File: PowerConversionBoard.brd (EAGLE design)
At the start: 152.4 x 76.2 mm, 48 parts, among them U1 LM2678, U2 LM2678

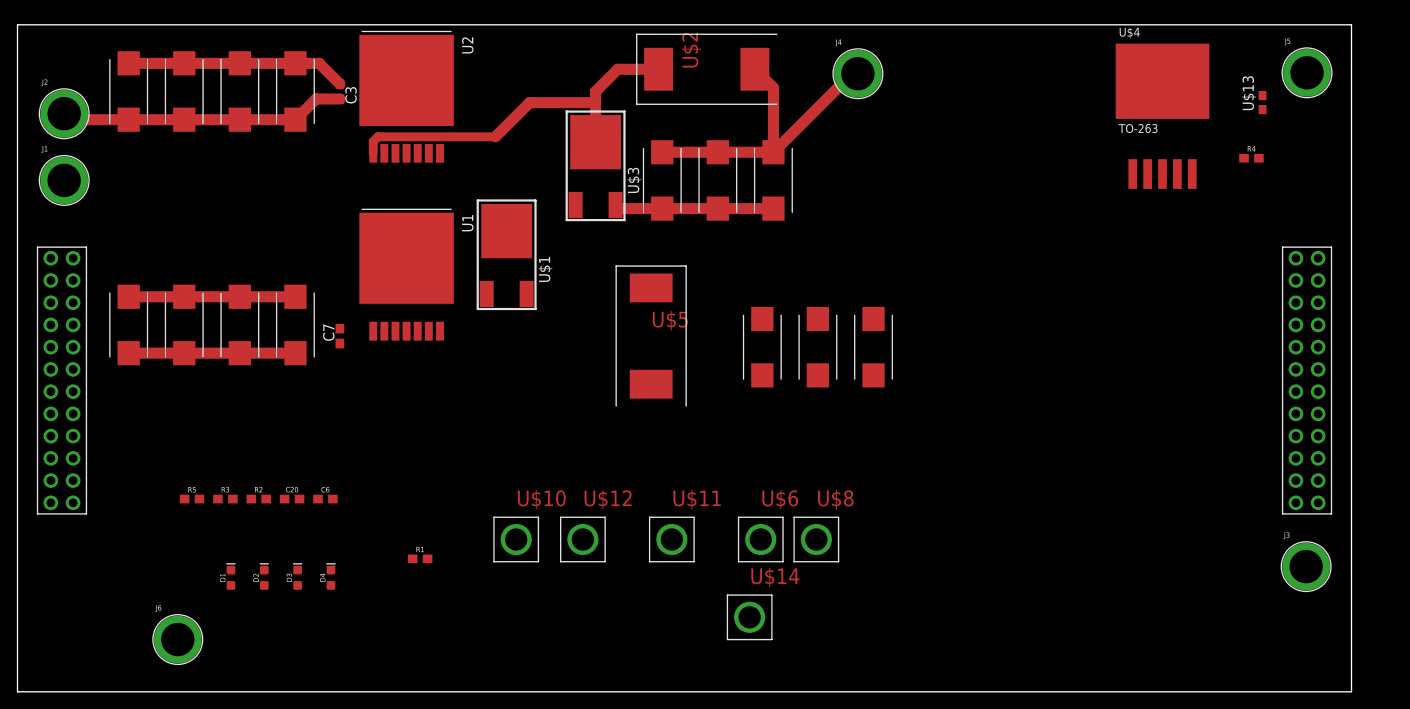
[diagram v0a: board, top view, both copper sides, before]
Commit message: Did some stuff
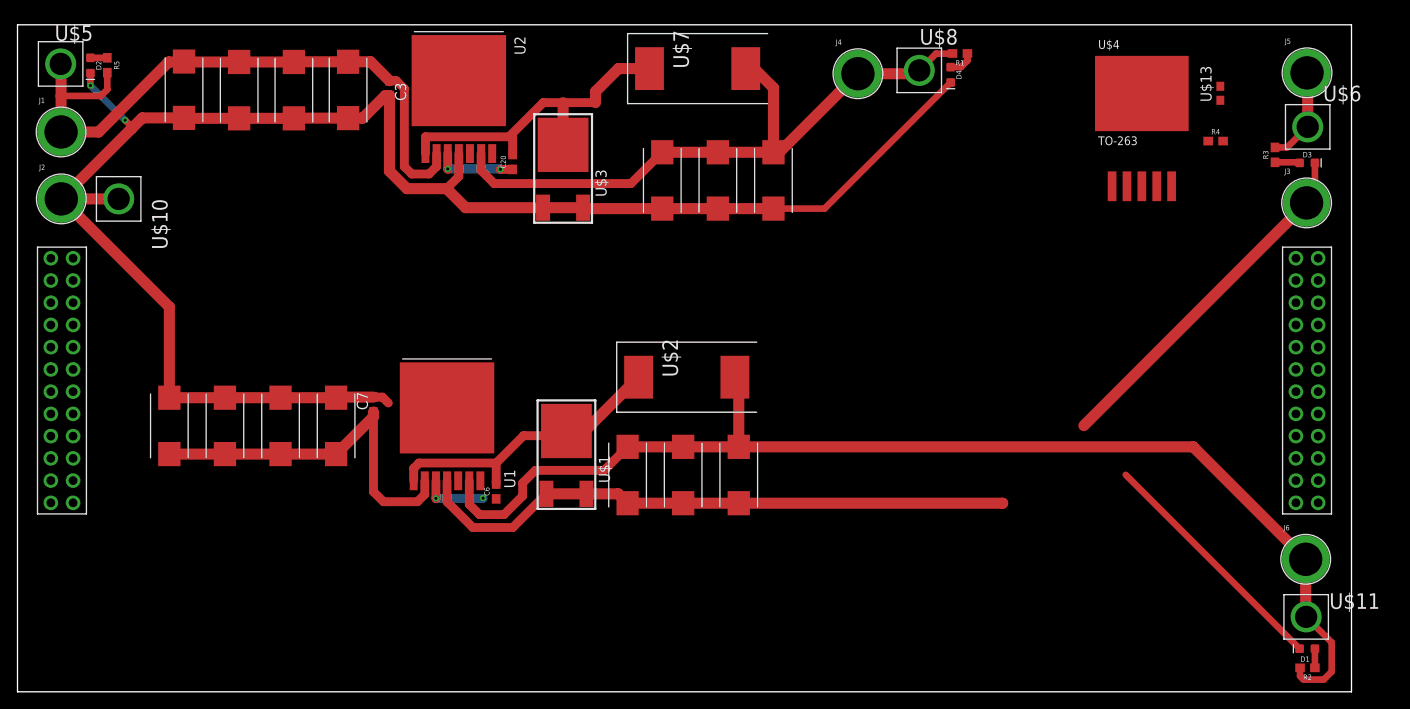
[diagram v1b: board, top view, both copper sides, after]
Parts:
- removed U$12, U$14: TP, TP:TP
- added U$7: HCM1305, HCM1305:HCM1305
- U$5: value HCM1305 -> TP; device HCM1305:HCM1305 -> TP:TP
- moved J6 129.2 mm to (147.2, 15.1)
- moved R3 126.2 mm to (143.7, 61.3), turned to 90 degrees
- moved D3 124.7 mm to (147.3, 60.4), turned to 0 degrees
- moved D1 123.2 mm to (147.3, 4.93), turned to 180 degrees
- moved R2 121.4 mm to (147.4, 2.74), turned to 180 degrees
- moved D4 91.2 mm to (106.6, 70.5), turned to 270 degrees
- moved R1 84.5 mm to (107.7, 72.9), turned to 180 degrees
- moved U$6 78.3 mm to (147.4, 64.5)
- moved U$5 74.3 mm to (4.93, 71.7)
- moved U$11 73.0 mm to (147.2, 8.56)
- moved D2 61.8 mm to (8.33, 71.6), turned to 270 degrees
- moved U$10 59.8 mm to (11.6, 56.3), turned to 270 degrees
- moved U$8 54.9 mm to (103.0, 71.0)
- moved R5 50.5 mm to (10.3, 71.6), turned to 270 degrees
- moved C20 46.0 mm to (56.6, 60.5), turned to 90 degrees
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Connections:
- net +12V: now also U$5.P$1; no longer U$12.P$1, U$14.P$1
- net +5V: now also U$11.P$1, U$2.2; no longer U$10.P$1, U$5.2
- net +5V_3.3V: now also U$7.2; no longer U$2.2
- net GND: now also U$10.P$1; no longer U$11.P$1
- net N$1: now also U$2.1; no longer U$5.1
- net N$7: now also U$7.1; no longer U$2.1
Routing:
- net GND: track 70.0 -> 335.6 mm, vias 0 -> 2
- net +5V: track 0.00 -> 135.5 mm
- net +12V: track 25.1 -> 73.9 mm
- net +5V_3.3V: track 36.4 -> 74.7 mm
- net N$1: track 0.00 -> 33.8 mm
- net N$20: track 19.1 -> 43.0 mm
- net +3.3V: track 0.00 -> 10.9 mm
- net N$2: track 0.00 -> 9.30 mm, vias 0 -> 2
- net N$3: track 0.00 -> 7.44 mm, vias 0 -> 1
- net N$7: track 42.6 -> 38.7 mm
- net N$6: track 0.00 -> 3.05 mm
- net N$5: track 0.00 -> 2.83 mm
- net N$8: track 0.00 -> 2.19 mm
- net N$4: track 0.00 -> 1.93 mm
